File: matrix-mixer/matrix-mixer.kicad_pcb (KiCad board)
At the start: 2 copper layers, 58.4 x 108 mm, 50 parts, among them IC1 LM324N, J1 EURO_HEADER_10pin

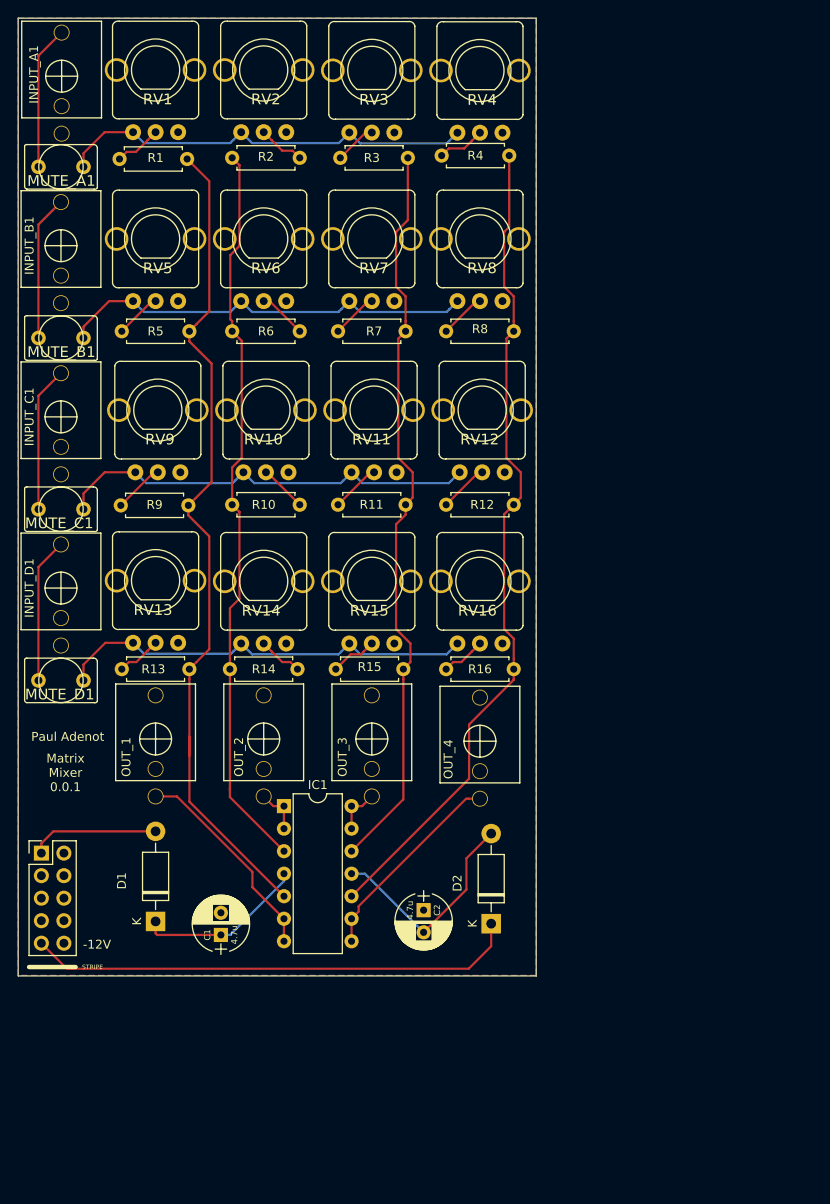
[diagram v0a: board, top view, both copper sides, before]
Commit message: version sent to fab
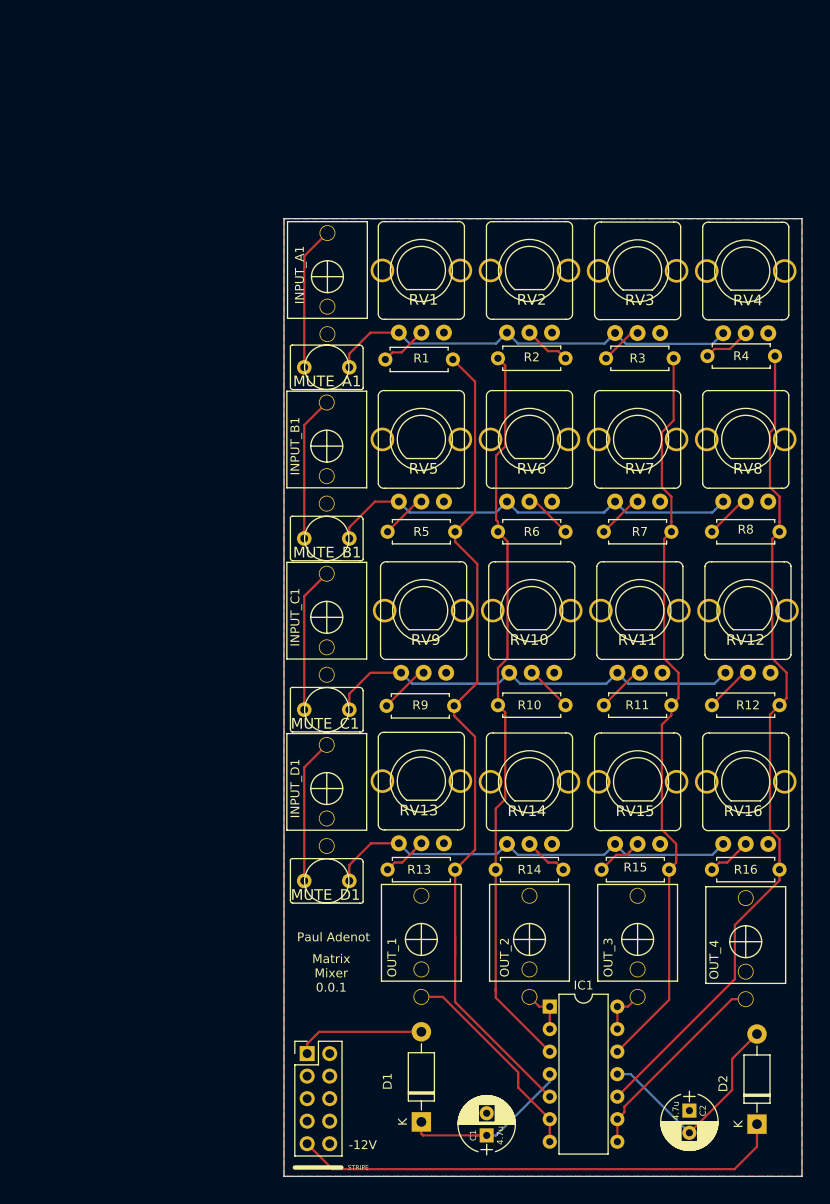
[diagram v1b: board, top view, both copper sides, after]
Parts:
- moved OUT_4 37.5 mm to (72.6, 98.6)
- moved C2 37.5 mm to (66.3, 117.6)
- moved D2 37.5 mm to (73.9, 119.1)
- moved J1 37.5 mm to (27.9, 121.9)
- moved R11 37.5 mm to (56.6, 71.9)
- moved R12 37.5 mm to (68.8, 71.9)
- moved R13 37.5 mm to (32.3, 90.4)
- moved R14 37.5 mm to (52.1, 90.4)
- moved R16 37.5 mm to (68.8, 90.4)
- moved R9 37.5 mm to (32.1, 72.0)
- moved RV10 37.5 mm to (48.5, 61.2)
- moved RV11 37.5 mm to (60.7, 61.2)
- moved RV16 37.5 mm to (72.6, 80.5)
- moved RV4 37.5 mm to (72.6, 22.9)
- moved RV8 37.5 mm to (72.6, 41.9)
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
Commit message: matrix 0.0.2 but not routed
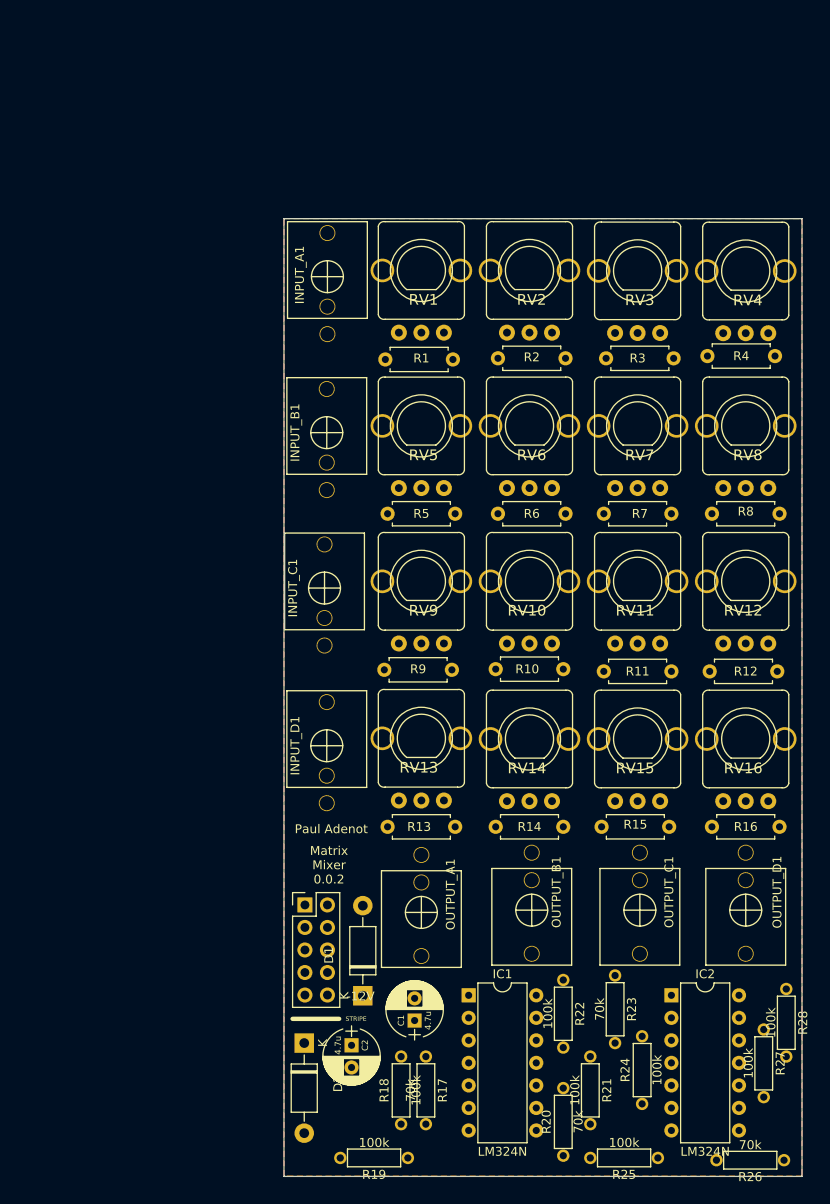
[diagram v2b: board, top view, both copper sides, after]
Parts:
- removed MUTE_A1, MUTE_B1, MUTE_C1, MUTE_D1: SW_SPST, 4ms-footprints:SPST-SUB
- added IC2: LM324N, 4ms_Package_DIP:DIP-14_W7.62mm, F.Cu at (64.3, 104.6)
- added R17: 70k, 4ms_Resistor:R_Axial_DIN0207_L6.3mm_D2.5mm_P7.62mm_Horizontal, F.Cu at (36.6, 115.3)
- added R18: 100k, 4ms_Resistor:R_Axial_DIN0207_L6.3mm_D2.5mm_P7.62mm_Horizontal, F.Cu at (33.8, 115.3)
- added R19: 100k, 4ms_Resistor:R_Axial_DIN0207_L6.3mm_D2.5mm_P7.62mm_Horizontal, F.Cu at (30.7, 122.9)
- added R20: 70k, 4ms_Resistor:R_Axial_DIN0207_L6.3mm_D2.5mm_P7.62mm_Horizontal, F.Cu at (52.1, 118.9)
- added R21: 100k, 4ms_Resistor:R_Axial_DIN0207_L6.3mm_D2.5mm_P7.62mm_Horizontal, F.Cu at (55.1, 115.3)
- added R22: 100k, 4ms_Resistor:R_Axial_DIN0207_L6.3mm_D2.5mm_P7.62mm_Horizontal, F.Cu at (52.1, 106.7)
- added R23: 70k, 4ms_Resistor:R_Axial_DIN0207_L6.3mm_D2.5mm_P7.62mm_Horizontal, F.Cu at (57.9, 106.2)
- added R24: 100k, 4ms_Resistor:R_Axial_DIN0207_L6.3mm_D2.5mm_P7.62mm_Horizontal, F.Cu at (61.0, 113.0)
- added R25: 100k, 4ms_Resistor:R_Axial_DIN0207_L6.3mm_D2.5mm_P7.62mm_Horizontal, F.Cu at (58.9, 122.9)
- added R26: 70k, 4ms_Resistor:R_Axial_DIN0207_L6.3mm_D2.5mm_P7.62mm_Horizontal, F.Cu at (73.2, 123.2)
- added R27: 100k, 4ms_Resistor:R_Axial_DIN0207_L6.3mm_D2.5mm_P7.62mm_Horizontal, F.Cu at (74.7, 112.3)
- added R28: 100k, 4ms_Resistor:R_Axial_DIN0207_L6.3mm_D2.5mm_P7.62mm_Horizontal, F.Cu at (77.2, 107.7)
- moved D2 51.9 mm to (22.9, 110.0), turned to 270 degrees
- moved C2 38.8 mm to (28.2, 110.2)
- moved J1 16.8 mm to (27.7, 105.2)
- moved D1 15.7 mm to (29.5, 104.6)
- moved C1 15.3 mm to (35.3, 107.4)
- moved IC1 9.23 mm to (41.4, 104.6)
- moved INPUT_D1 4.83 mm to (25.4, 76.5)
- moved R13 4.83 mm to (32.3, 85.6)
- moved R14 4.83 mm to (52.1, 85.6)
- moved R15 4.83 mm to (56.4, 85.6)
- moved R16 4.83 mm to (68.8, 85.6)
- moved RV13 4.83 mm to (36.1, 75.6)
- moved RV14 4.83 mm to (48.3, 75.7)
- moved RV15 4.83 mm to (60.5, 75.7)
- moved RV16 4.83 mm to (72.6, 75.7)
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- renumbered OUT_1 to OUTPUT_A1, OUT_2 to OUTPUT_B1, OUT_3 to OUTPUT_C1, OUT_4 to OUTPUT_D1
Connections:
- IC1 pad 10: Net-(IC1-Pad10) -> GND
- IC1 pad 12: Net-(IC1-Pad12) -> GND
- IC1 pad 14: Net-(IC1-Pad13) -> Net-(IC1-Pad14)
- IC1 pad 2: Net-(IC1-Pad1) -> Net-(IC1-Pad2)
- IC1 pad 3: Net-(IC1-Pad3) -> GND
- IC1 pad 5: Net-(IC1-Pad5) -> GND
- IC1 pad 7: Net-(IC1-Pad6) -> Net-(IC1-Pad7)
- IC1 pad 9: Net-(IC1-Pad8) -> Net-(IC1-Pad9)
- INPUT_A1 pad 1: Net-(INPUT_A1-Pad1) -> (no net)
- INPUT_B1 pad 1: Net-(INPUT_B1-Pad1) -> (no net)
- INPUT_C1 pad 1: Net-(INPUT_C1-Pad1) -> (no net)
- INPUT_D1 pad 1: Net-(INPUT_D1-Pad1) -> (no net)
- J1 pad 10: Net-(J1-Pad10) -> (no net)
- J1 pad 2: Net-(J1-Pad2) -> (no net)
- OUTPUT_A1 pad 1: Net-(IC1-Pad6) -> (no net)
- OUTPUT_A1 pad 3: Net-(J2-Pad3) -> Net-(IC1-Pad7)
- OUTPUT_B1 pad 1: Net-(IC1-Pad1) -> (no net)
- OUTPUT_B1 pad 3: Net-(J3-Pad3) -> Net-(IC1-Pad14)
- OUTPUT_C1 pad 1: Net-(IC1-Pad13) -> (no net)
- OUTPUT_D1 pad 1: Net-(IC1-Pad8) -> (no net)
- R1 pad 2: Net-(IC1-Pad5) -> Net-(IC1-Pad2)
- R10 pad 2: Net-(IC1-Pad3) -> Net-(IC1-Pad9)
- R11 pad 2: Net-(IC1-Pad12) -> Net-(IC2-Pad2)
- R12 pad 2: Net-(IC1-Pad10) -> Net-(IC2-Pad9)
- R13 pad 2: Net-(IC1-Pad5) -> Net-(IC1-Pad2)
- R14 pad 2: Net-(IC1-Pad3) -> Net-(IC1-Pad9)
- R15 pad 2: Net-(IC1-Pad12) -> Net-(IC2-Pad2)
- R16 pad 2: Net-(IC1-Pad10) -> Net-(IC2-Pad9)
- R2 pad 2: Net-(IC1-Pad3) -> Net-(IC1-Pad9)
- R3 pad 2: Net-(IC1-Pad12) -> Net-(IC2-Pad2)
- R4 pad 2: Net-(IC1-Pad10) -> Net-(IC2-Pad9)
- R5 pad 2: Net-(IC1-Pad5) -> Net-(IC1-Pad2)
- R6 pad 2: Net-(IC1-Pad3) -> Net-(IC1-Pad9)
- R7 pad 2: Net-(IC1-Pad12) -> Net-(IC2-Pad2)
- R8 pad 2: Net-(IC1-Pad10) -> Net-(IC2-Pad9)
- R9 pad 2: Net-(IC1-Pad5) -> Net-(IC1-Pad2)
- RV1 pad 1: Net-(MUTE_A1-Pad2) -> GND
- RV1 pad 3: GND -> Net-(INPUT_A1-Pad3)
- RV10 pad 1: Net-(MUTE_C1-Pad2) -> GND
- RV10 pad 3: GND -> Net-(INPUT_C1-Pad3)
- RV11 pad 1: Net-(MUTE_C1-Pad2) -> GND
- RV11 pad 3: GND -> Net-(INPUT_C1-Pad3)
- RV12 pad 1: Net-(MUTE_C1-Pad2) -> GND
- RV12 pad 3: GND -> Net-(INPUT_C1-Pad3)
- RV13 pad 1: Net-(MUTE_D1-Pad2) -> GND
- RV13 pad 3: GND -> Net-(INPUT_D1-Pad3)
- RV14 pad 1: Net-(MUTE_D1-Pad2) -> GND
- RV14 pad 3: GND -> Net-(INPUT_D1-Pad3)
- RV15 pad 1: Net-(MUTE_D1-Pad2) -> GND
- RV15 pad 3: GND -> Net-(INPUT_D1-Pad3)
- RV16 pad 1: Net-(MUTE_D1-Pad2) -> GND
- RV16 pad 3: GND -> Net-(INPUT_D1-Pad3)
- RV2 pad 1: Net-(MUTE_A1-Pad2) -> GND
- RV2 pad 3: GND -> Net-(INPUT_A1-Pad3)
- RV3 pad 1: Net-(MUTE_A1-Pad2) -> GND
- RV3 pad 3: GND -> Net-(INPUT_A1-Pad3)
- RV4 pad 1: Net-(MUTE_A1-Pad2) -> GND
- RV4 pad 3: GND -> Net-(INPUT_A1-Pad3)
- RV5 pad 1: Net-(MUTE_B1-Pad2) -> GND
- RV5 pad 3: GND -> Net-(INPUT_B1-Pad3)
- RV6 pad 1: Net-(MUTE_B1-Pad2) -> GND
- RV6 pad 3: GND -> Net-(INPUT_B1-Pad3)
- RV7 pad 1: Net-(MUTE_B1-Pad2) -> GND
- RV7 pad 3: GND -> Net-(INPUT_B1-Pad3)
- RV8 pad 1: Net-(MUTE_B1-Pad2) -> GND
- RV8 pad 3: GND -> Net-(INPUT_B1-Pad3)
- RV9 pad 1: Net-(MUTE_C1-Pad2) -> GND
- RV9 pad 3: GND -> Net-(INPUT_C1-Pad3)
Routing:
- net Net-(IC1-Pad5): track 95.7 -> 0.00 mm
- net Net-(IC1-Pad10): track 94.0 -> 0.00 mm
- net Net-(IC1-Pad12): track 84.4 -> 0.00 mm
- net Net-(IC1-Pad3): track 83.5 -> 0.00 mm
- net Net-(D2-Pad1): track 55.5 -> 0.00 mm
- net Net-(MUTE_C1-Pad2): track 48.2 -> 0.00 mm
- net Net-(MUTE_D1-Pad2): track 48.0 -> 0.00 mm
- net Net-(MUTE_A1-Pad2): track 47.7 -> 0.00 mm
- net Net-(MUTE_B1-Pad2): track 47.7 -> 0.00 mm
- net /VEE: track 25.2 -> 0.00 mm
- net Net-(IC1-Pad6): track 23.7 -> 0.00 mm
- net Net-(IC1-Pad8): track 23.0 -> 0.00 mm
- net /VCC: track 19.3 -> 0.00 mm
- net Net-(INPUT_D1-Pad3): track 16.4 -> 0.00 mm
- net Net-(INPUT_C1-Pad3): track 16.4 -> 0.00 mm
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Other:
- board text added: "Matrix Mixer 0.0.2"
- board text removed: "Matrix Mixer 0.0.1"
